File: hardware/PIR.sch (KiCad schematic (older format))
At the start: 57 parts, among them U10 IRA-S210ST01, U11 OPA349SA/3K, U13 OPA349SA/3K, U14 TLV369IDCKT, U15 TLV369IDCKT, U16 TLV3691IDCKR, U17 TLV3691IDCKR, U9 IRA-S210ST01

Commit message: updatE
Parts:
- U11: footprint TO_SOT_Packages_SMD:SOT-23-5 -> TO_SOT_Packages_SMD:SOT-23-5_HandSoldering
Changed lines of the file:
@@
 F 0 "U11" H 6450 3950 50  0000 L CNN
 F 1 "OPA349SA/3K" H 6450 3850 50  0000 L CNN
-F 2 "TO_SOT_Packages_SMD:SOT-23-5" H 6450 3550 50  0001 L CNN
+F 2 "TO_SOT_Packages_SMD:SOT-23-5_HandSoldering" H 6450 3550 50  0001 L CNN
 F 3 "https://www.digikey.com/product-detail/en/texas-instruments/OPA349NA-3K/296-39127-1-ND/5143141" H 6900 3300 50  0001 C CNN
 F 4 "OPA349NA/3K" H 6550 4050 60  0001 C CNN "Part Number"

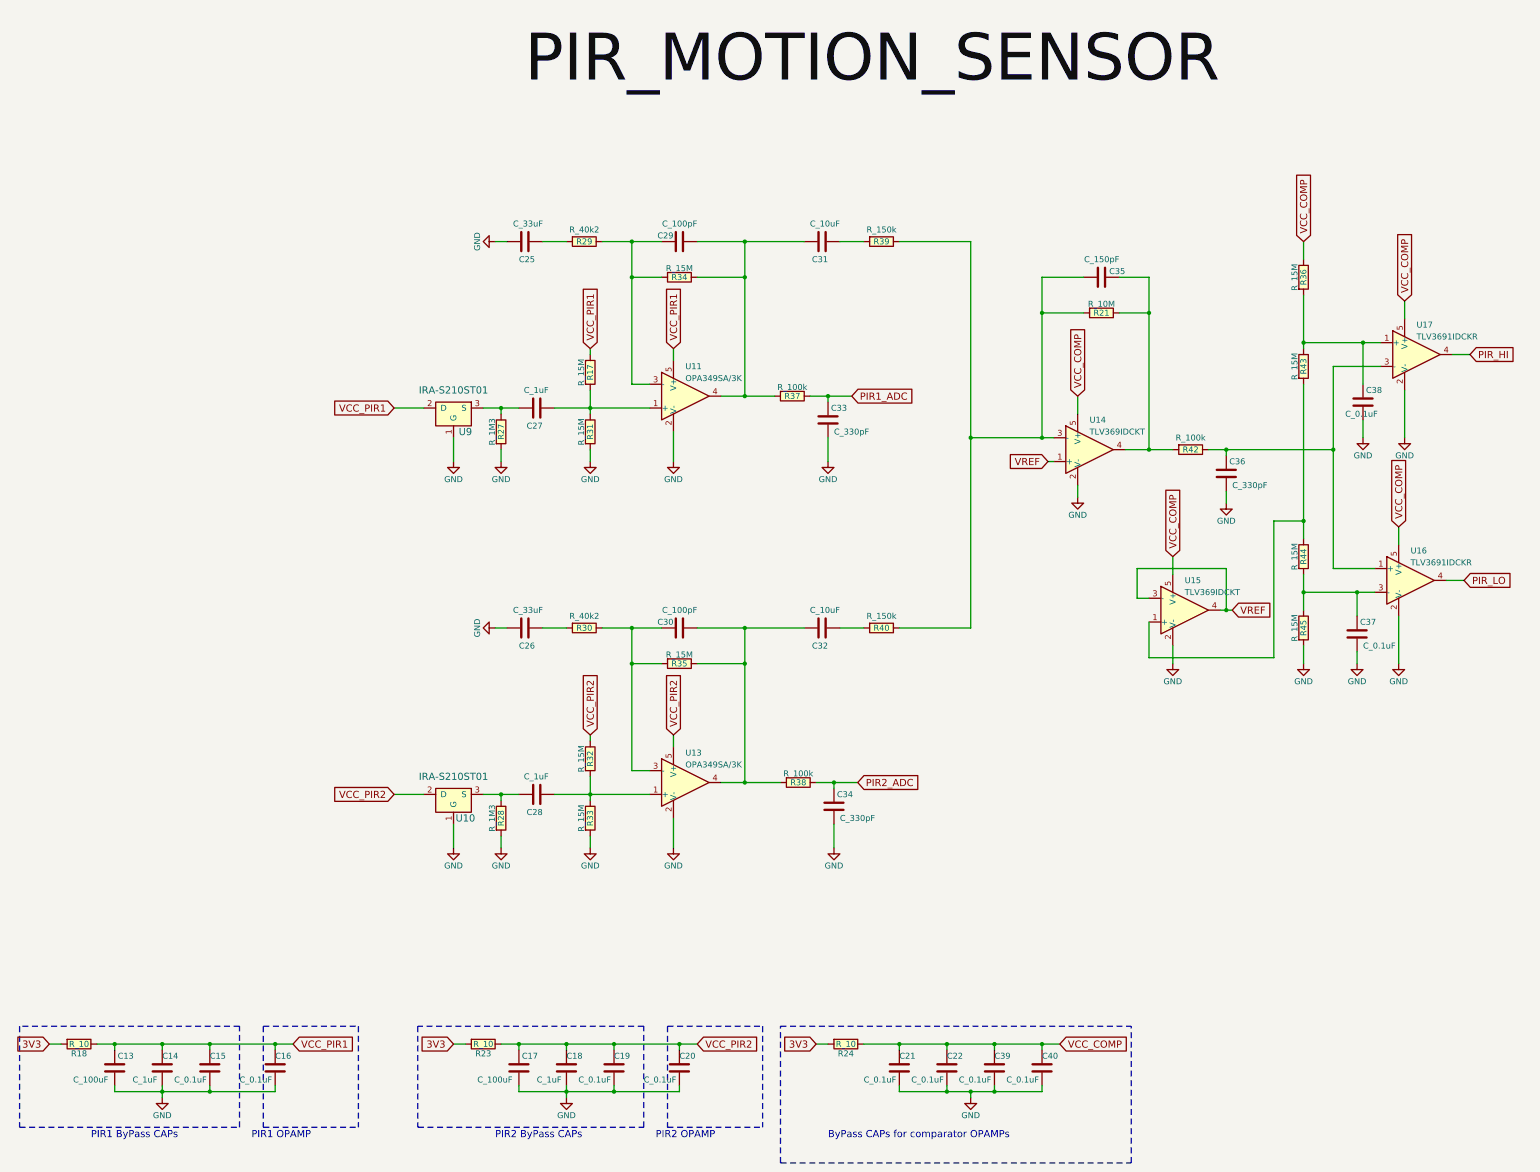
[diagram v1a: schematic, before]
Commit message: update
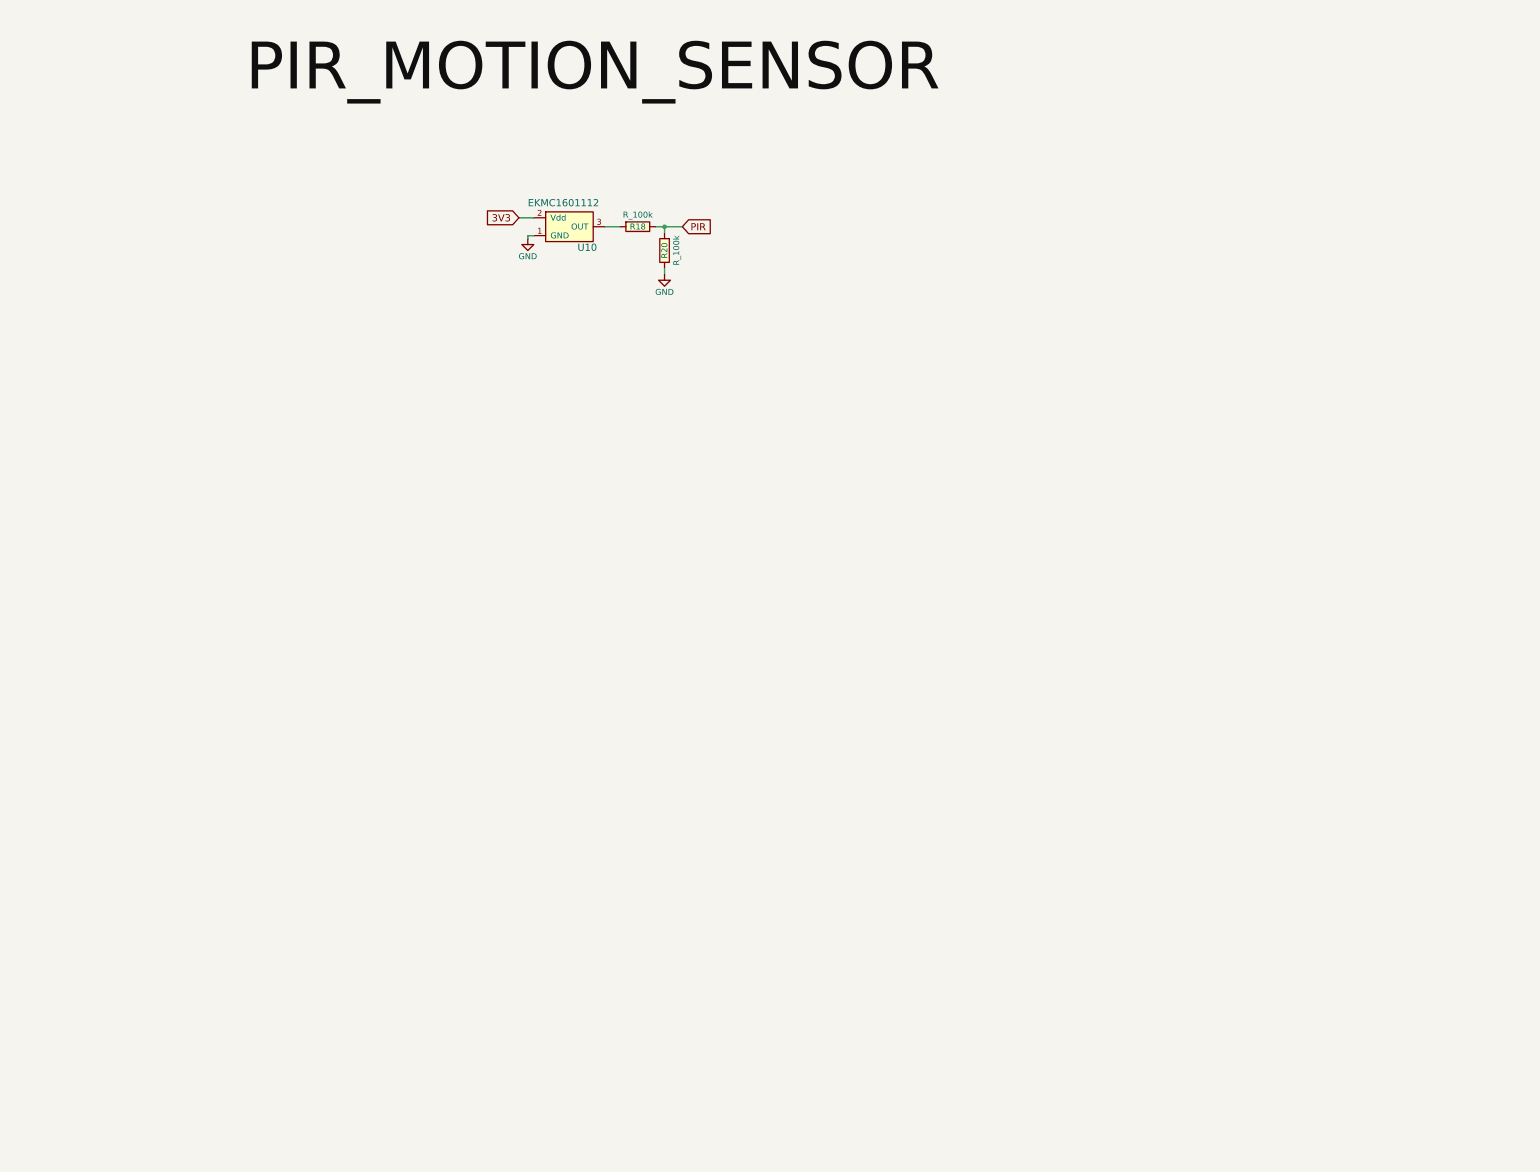
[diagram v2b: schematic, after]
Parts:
- removed C13: C_100uF, Capacitors_SMD:C_0603_HandSoldering, symbol C_100uF
- removed C14, C18, C27, C28: C_1uF, Capacitors_SMD:C_0603_HandSoldering, symbol C_1uF
- removed C15, C16, C19, C20, C21, C22, C37, C38, C39, C40: C_0.1uF, Capacitors_SMD:C_0603_HandSoldering, symbol C_0.1uF
- removed C17: C_100uF, Capacitors_SMD:C_1206_HandSoldering, symbol C_100uF
- removed C25, C26: C_33uF, Capacitors_SMD:C_0805_HandSoldering, symbol C_33uF
- removed C29, C30: C_100pF, Capacitors_SMD:C_0603_HandSoldering, symbol C_100pF
- removed C31, C32: C_10uF, Capacitors_SMD:C_0603_HandSoldering, symbol C_10uF
- removed C33, C34, C36: C_330pF, Capacitors_SMD:C_0603_HandSoldering, symbol C_330pF
- removed C35: C_150pF, Capacitors_SMD:C_0603_HandSoldering, symbol C_150pF
- removed R17, R31, R32, R33, R34, R35, R36, R43, R44, R45: R_15M, Resistors_SMD:R_0603_HandSoldering, symbol R_15M
- removed R18, R23, R24: R_10, Resistors_SMD:R_0603_HandSoldering, symbol R_10
- removed R21: R_10M, Resistors_SMD:R_0805_HandSoldering, symbol R_10M
- removed R27, R28: R_1M3, Resistors_SMD:R_0603_HandSoldering, symbol R_1M3
- removed R29, R30: R_40k2, Resistors_SMD:R_0603_HandSoldering, symbol R_40k2
- removed R37, R38, R42: R_100k, Resistors_SMD:R_0603_HandSoldering, symbol R_100k
- removed R39, R40: R_150k, Resistors_SMD:R_0603_HandSoldering, symbol R_150k
- removed U10, U9: IRA-S210ST01, open-automation:IRA-S210ST01, symbol IRA-S210ST01
- removed U11, U13: OPA349SA/3K, TO_SOT_Packages_SMD:SOT-23-5_HandSoldering, symbol OPA349SA/3K
- removed U14, U15: TLV369IDCKT, TO_SOT_Packages_SMD:SOT-23-5_HandSoldering, symbol TLV369IDCKT
- removed U16, U17: TLV3691IDCKR, TO_SOT_Packages_SMD:SOT-353_SC-70-5_Handsoldering, symbol TLV3691IDCKR
- added R18, R20: R_100k, Resistors_SMD:R_0603_HandSoldering, symbol R_100k
- added U10: EKMC1601112, open-automation:EKMC1601112, symbol EKMC1601112
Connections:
- net 3V3: now also U10.2 (Vdd)
- net GND: now also R20.1, U10.1 (GND)
- new net: R18.2, U10.3 (OUT)
- new net PIR: R18.1, R20.2
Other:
- note removed: "ByPass CAPs for comparator OPAMPs"
- note removed: "PIR1 ByPass CAPs"
- note removed: "PIR1 OPAMP"
- note removed: "PIR2 ByPass CAPs"
- note removed: "PIR2 OPAMP"

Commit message: update
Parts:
- R18, R20: symbol R_100k -> liger-rescue:R_100k
- U10: symbol EKMC1601112 -> liger-rescue:EKMC1601112
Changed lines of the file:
@@
-EESchema Schematic File Version 2
-LIBS:power
-LIBS:device
-LIBS:transistors
-LIBS:conn
-LIBS:linear
-LIBS:regul
-LIBS:74xx
-LIBS:cmos4000
-LIBS:adc-dac
-LIBS:memory
-LIBS:xilinx
-LIBS:microcontrollers
-LIBS:dsp
-LIBS:microchip
-LIBS:analog_switches
-LIBS:motorola
-LIBS:texas
-LIBS:intel
-LIBS:audio
-LIBS:interface
-LIBS:digital-audio
-LIBS:philips
-LIBS:display
-LIBS:cypress
-LIBS:siliconi
-LIBS:opto
-LIBS:atmel
-LIBS:contrib
-LIBS:valves
-LIBS:open-automation
+EESchema Schematic File Version 4
 LIBS:liger-cache
-EELAYER 25 0
+EELAYER 26 0
 EELAYER END
 $Descr A4 11693 8268
@@
 PIR
 $Comp
-L GND #PWR029
+L power:GND #PWR029
 U 1 1 59B7E3DB
 P 5125 2375
@@
 3V3
 $Comp
-L R_100k R18
+L liger-rescue:R_100k R18
 U 1 1 5A160B80
 P 6050 2275
@@
 $EndComp
 $Comp
-L R_100k R20
+L liger-rescue:R_100k R20
 U 1 1 5A1610DC
 P 6275 2475
@@
 	6275 2275 6275 2325
 $Comp
-L GND #PWR030
+L power:GND #PWR030
 U 1 1 5A1624EE
 P 6275 2675
@@
 Connection ~ 6275 2275
 $Comp
-L EKMC1601112 U10
+L liger-rescue:EKMC1601112 U10
 U 1 1 5A1702E3
 P 5425 2275
